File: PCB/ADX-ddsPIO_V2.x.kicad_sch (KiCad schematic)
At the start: 77 parts, among them J1 Conn_Coaxial, J2 +12V, Q1 BS170, Q2 BS170, Q3 BS170, Q5 BS170, U1 L7805, U2 74LS244, U4 CD2003GB_GP, U5 SI4732-A10-GS, Y1 IF resonator

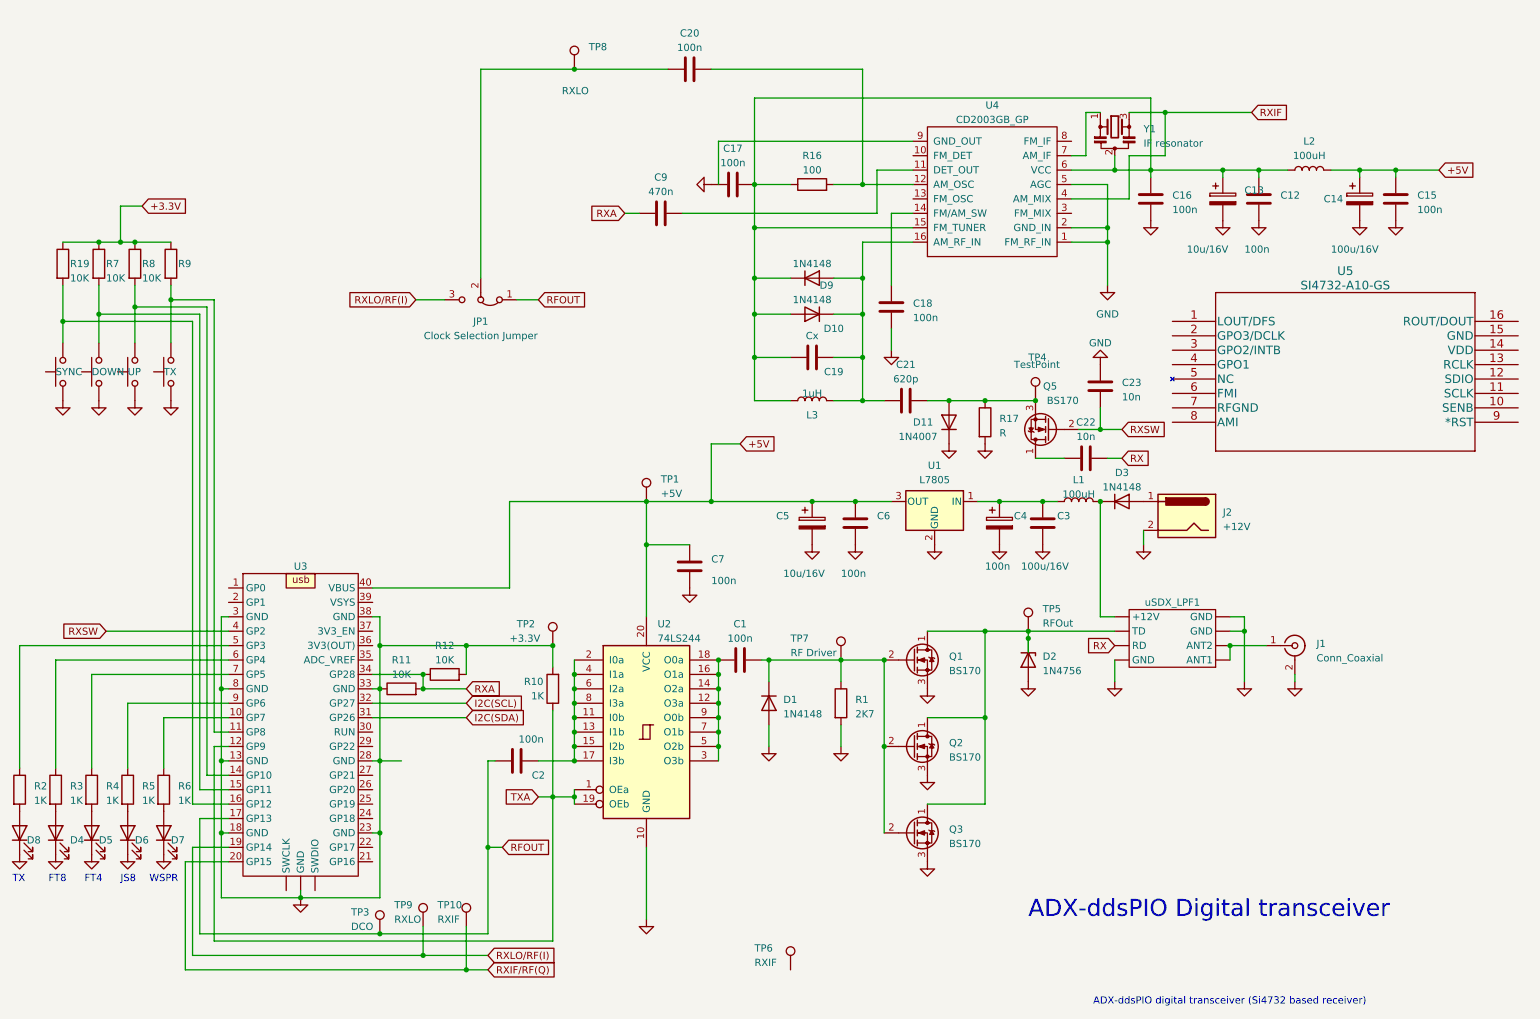
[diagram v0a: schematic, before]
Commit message: si4732_rp2040
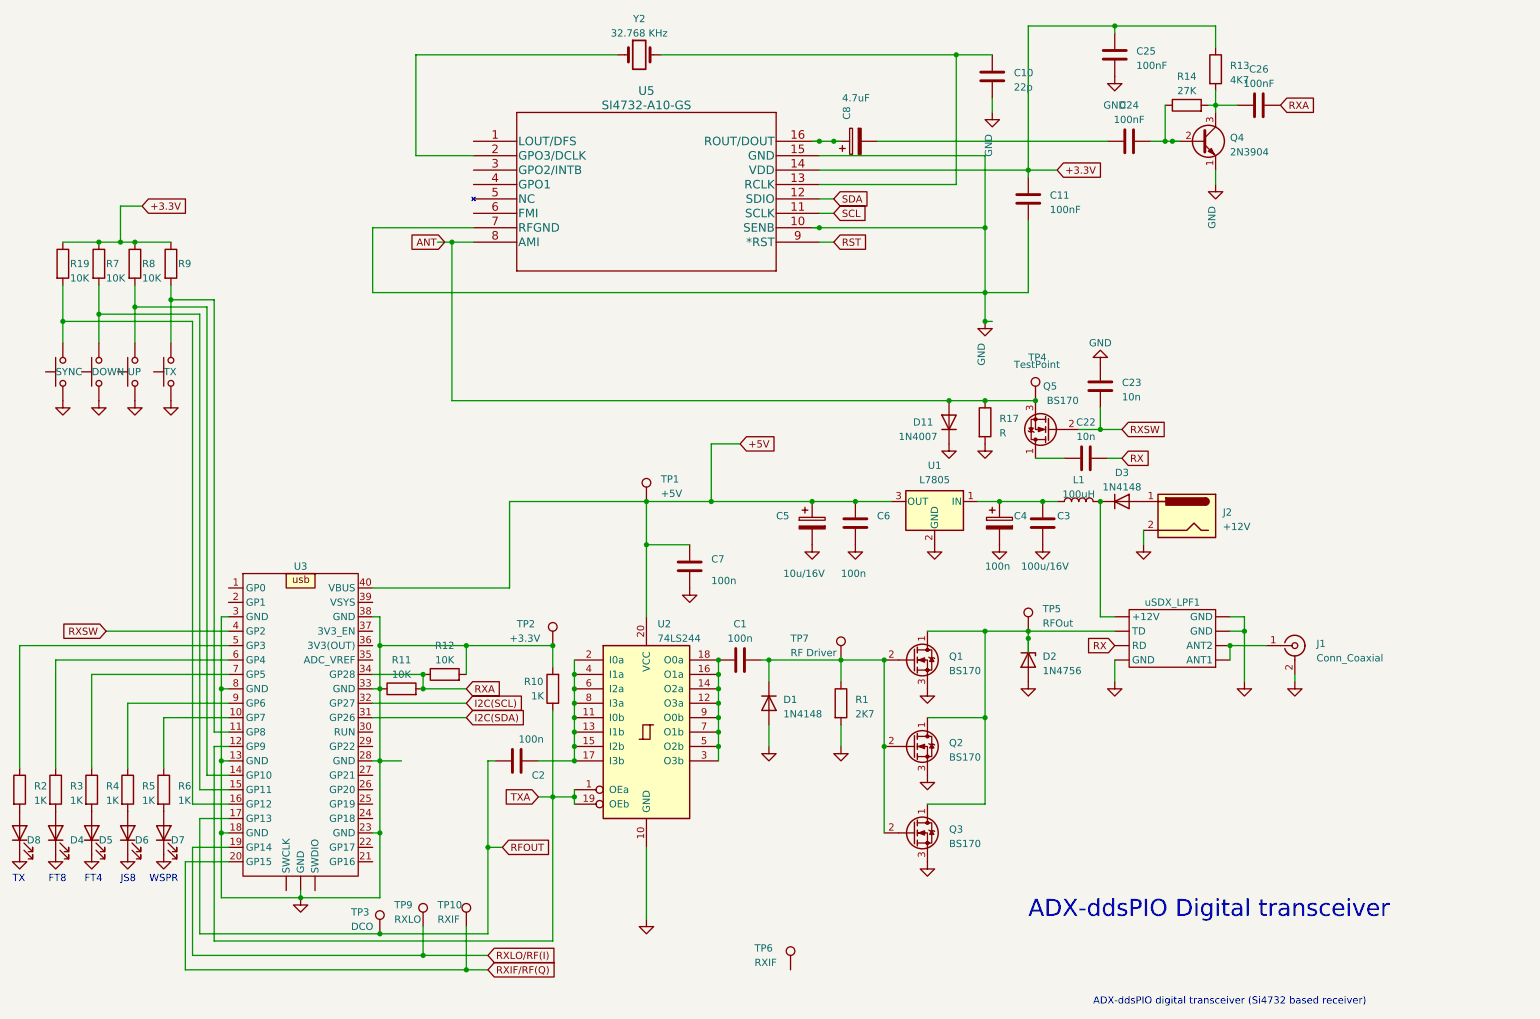
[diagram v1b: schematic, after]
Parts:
- removed C12, C15, C16, C17, C18, C20: 100n, symbol Device:C
- removed C13: 10u/16V, symbol Device:C_Polarized
- removed C14: 100u/16V, symbol Device:C_Polarized
- removed C19: Cx, symbol Device:C
- removed C21: 620p, symbol Device:C
- removed C9: 470n, symbol Device:C
- removed D10, D9: 1N4148, Diode_THT:D_DO-35_SOD27_P7.62mm_Horizontal, symbol Diode:1N4148
- removed JP1: Clock Selection Jumper, symbol Jumper:Jumper_3_Bridged12
- removed L2: 100uH, symbol Device:L
- removed L3: 1uH, symbol Device:L
- removed R16: 100, symbol Device:R
- removed TP8: RXLO, symbol Connector:TestPoint
- removed U4: CD2003GB_GP, symbol CD2003 Library:CD2003GB_GP
- removed Y1: IF resonator, symbol Device:Resonator_Small
- added C10: 22p, symbol Device:C
- added C11, C24, C25, C26: 100nF, symbol Device:C
- added C8: 4.7uF, symbol Device:C_Polarized
- added Q4: 2N3904, Package_TO_SOT_THT:TO-92_Inline, symbol Transistor_BJT:2N3904
- added R13: 4K7, symbol Device:R
- added R14: 27K, symbol Device:R
- added Y2: 32.768 KHz, symbol Device:Crystal
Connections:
- net +3.3V: now also U5.14 (VDD), C11.1, C25.1, R13.1
- net GND: now also U5.10 (SENB), U5.15 (GND), U5.7 (RFGND), C10.2, C11.2, C25.2, Q4.1 (E)
- net RXA: now also C26.2
- net ANT: now reaches D11.2 (A), Q5.3 (S), R17.1, TP4.1
- net ANT: now also U5.8 (AMI)
- net SCL: now reaches U5.11 (SCLK)
- net SDA: now reaches U5.12 (SDIO)
- net at U5.13 (RCLK): now also C10.1, Y2.2
- net at U5.16 (ROUT/DOUT): now also C8.1
- net at U5.2 (GPO3/DCLK): now also Y2.1
- net RST: now reaches U5.9 (*RST)
- new net: C24.1, C8.2
- new net: C24.2, Q4.2 (B), R14.1
- new net: C26.1, Q4.3 (C), R13.2, R14.2
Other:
- moved on the sheet: U5

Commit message: ddsPIO-RDX
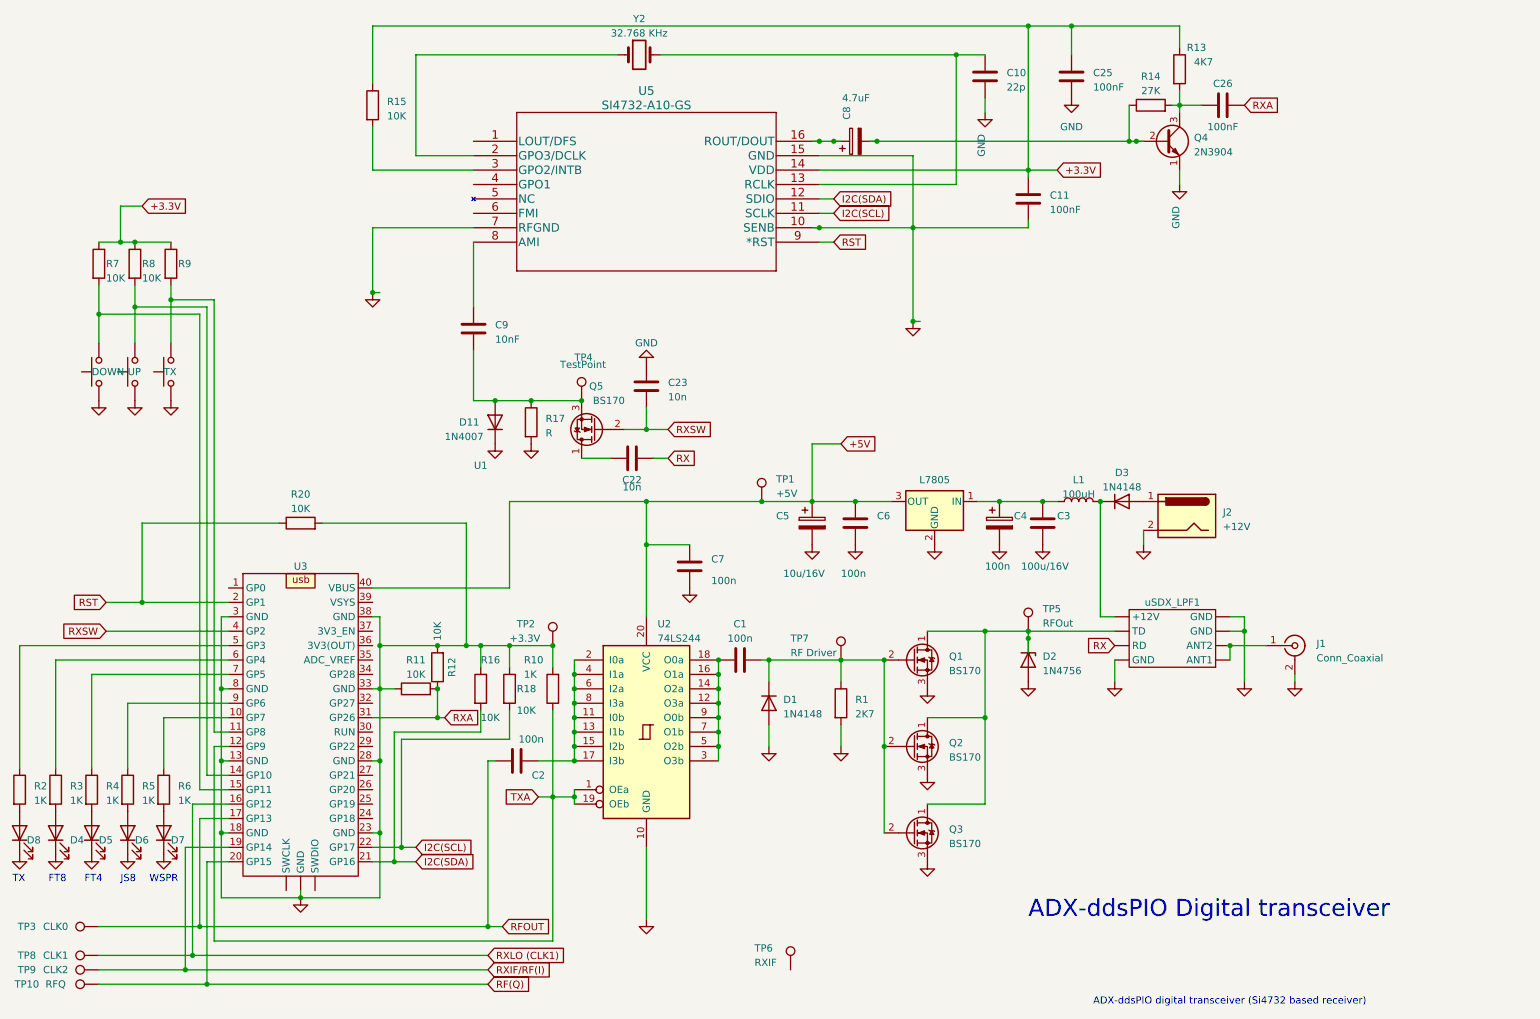
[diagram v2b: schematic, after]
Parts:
- removed C24: 100nF, symbol Device:C
- removed R19: 10K, symbol Device:R
- removed SYNC: SW_MEC_5G, symbol Switch:SW_MEC_5G
- added C9: 10nF, symbol Device:C
- added R15, R16, R18, R20: 10K, symbol Device:R
- added TP8: CLK1, symbol Connector:TestPoint
- TP10: value RXIF -> RFQ
- TP3: value DCO -> CLK0
- TP9: value RXLO -> CLK2
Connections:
- net SCL is gone; now on net I2C(SCL): U5.11 (SCLK)
- net SDA is gone; now on net I2C(SDA): U5.12 (SDIO)
- net +3.3V: now also R15.1
- net GND: now also R16.1, R18.1, R20.2
- net I2C(SCL): now also U3.22 (GP17), R18.2; no longer U3.32 (GP27)
- net I2C(SDA): now also U3.21 (GP16), R16.2; no longer U3.31 (GP26)
- net RST: now also U3.2 (GP1), R20.1
- net RXA: now also U3.31 (GP26); no longer U3.34 (GP28)
- net RXLO (CLK1): now reaches U3.16 (GP12)
- net RXLO (CLK1): now also TP8.1
- net at C8.2: now also Q4.2 (B), R14.1
- net at U5.3 (GPO2/INTB): now also R15.2
- net ANT: no longer names the net of D11.2 (A), Q5.3 (S), R17.1, TP4.1
- net ANT: now also C9.2; no longer U5.8 (AMI)
- net RXIF/RF(Q) renamed RF(Q)
- net RXLO/RF(I) renamed RXIF/RF(I)
- new net: C9.1, U5.8 (AMI)
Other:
- moved on the sheet: C10, C22, C23, C25, C26, D11, Q4, Q5, R11, R12, R13, R14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
